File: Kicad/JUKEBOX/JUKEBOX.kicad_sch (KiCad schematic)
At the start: 34 parts, among them J1 Entrada 5V, J10 Fader volumen (B10K), J2 Salida 5V a P4 CIAA, J3 OLED SH1106 I2C, J4 RFID RC522, J5 Parlante respaldo (mono), J6 Alim. PAM8403, J7 Audio a PAM8403, J8 ULN2003 IN1-IN4, J9 ULN2003 alimentación, U1 DFPlayer_Mini, U2 24LC256

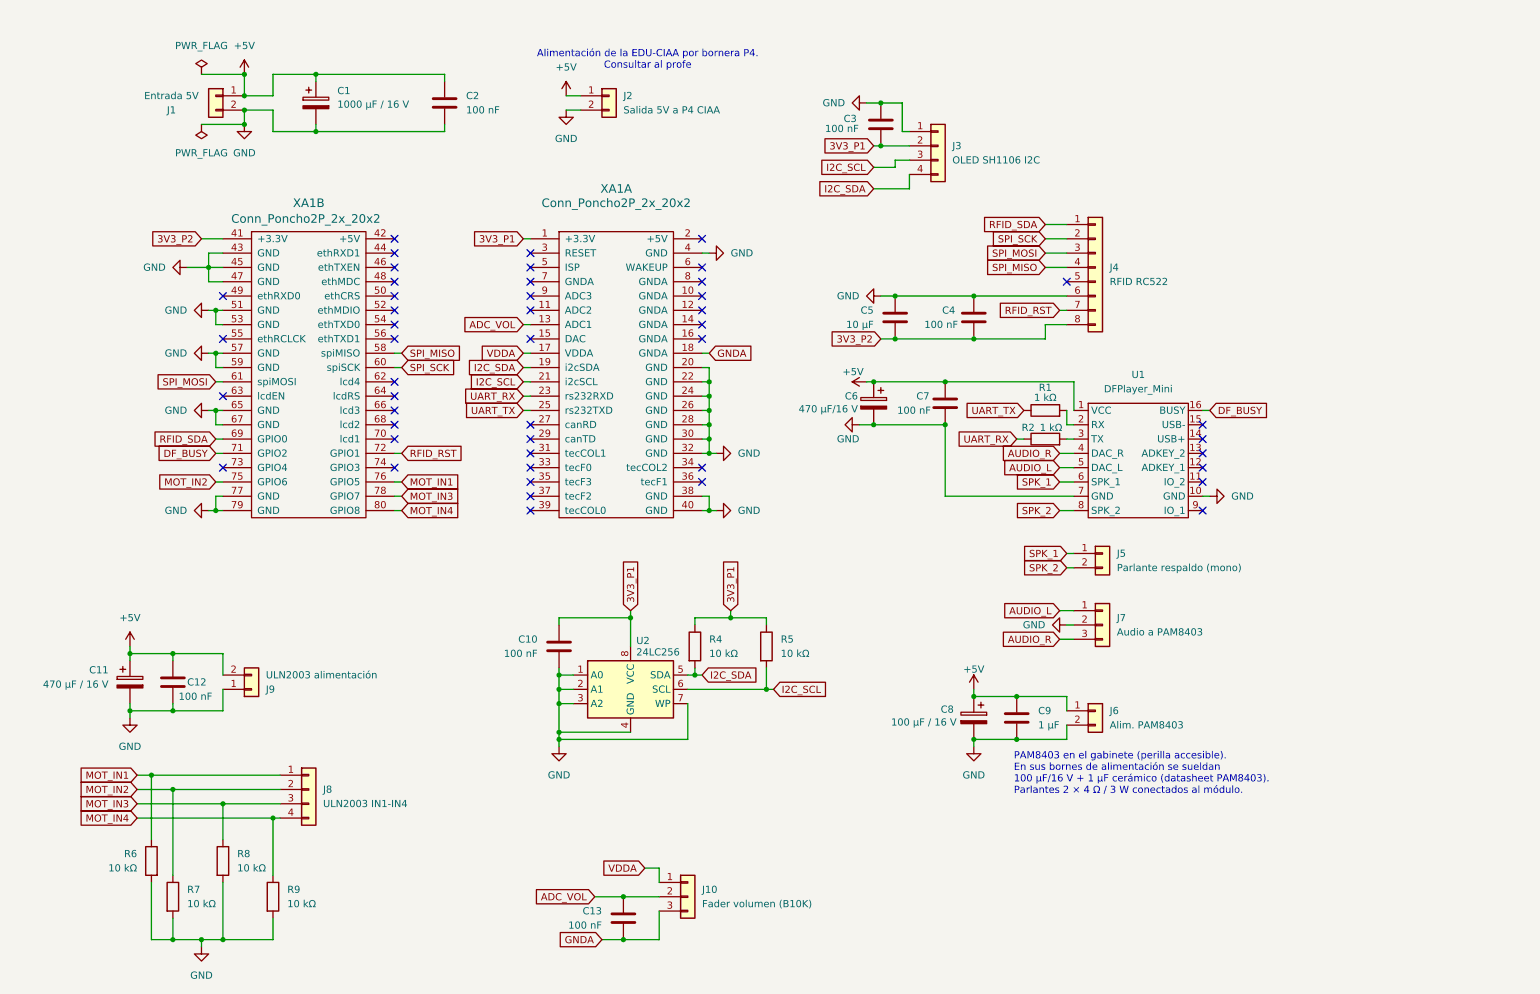
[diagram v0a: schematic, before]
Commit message: Actualizacion: neopixel + buffer 74AHCT125
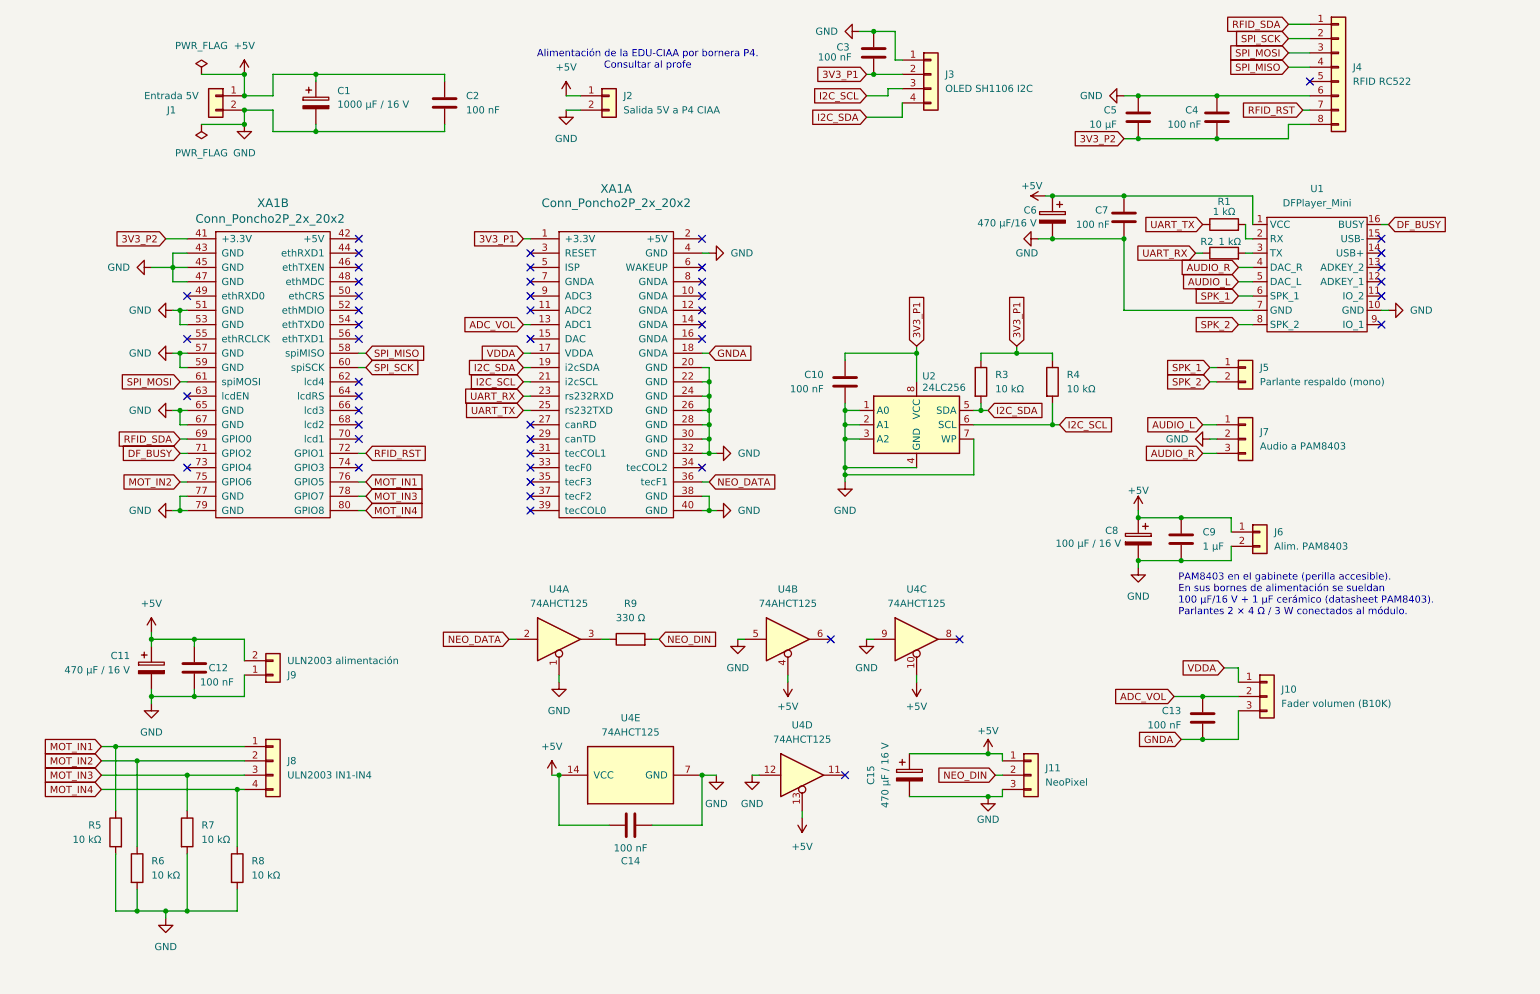
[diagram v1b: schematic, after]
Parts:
- added C14: 100 nF, symbol Device:C
- added C15: 470 µF / 16 V, symbol Device:C_Polarized
- added J11: NeoPixel, symbol Connector_Generic:Conn_01x03
- added R9: 330 Ω, symbol Device:R
- added U4: 74AHCT125, Package_CSP:Xilinx_CSG48_7.0x7.0mm_Layout7x7_P0.8mm, symbol 74xx:74AHCT125
- renumbered R4 to R3, R5 to R4, R6 to R5, R7 to R6, R8 to R7, R9 to R8
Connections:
- net +5V: now also C14.1, C15.1, J11.1 (Pin_1), U4.10, U4.13, U4.14 (VCC), U4.4
- net GND: now also C14.2, C15.2, J11.3 (Pin_3), U4.1, U4.12, U4.5, U4.7 (GND), U4.9
- net NEO_DATA: now reaches XA1.36 (tecF1)
- net NEO_DATA: now also U4.2
- new net: R9.1, U4.3
- new net NEO_DIN: J11.2 (Pin_2), R9.2
- no-connect marks 47 -> 49
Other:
- moved on the sheet: C10, C11, C12, C13, C3, C4, C5, C6, C7, C8, C9, J10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
